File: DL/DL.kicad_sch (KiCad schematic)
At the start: 39 parts, among them IC1 MCP6V96UT-E_OT, IC2 SCD42-D-R2, IC3 TGS3870-B00, J3 SD_Card, J4 Conn_01x05_Male, J5 Conn_01x05_Male, J6 Conn_01x05_Male, J7 Conn_01x05_Male, Q1 BSS84, Q2 2N7002, U1 SHT31-DIS, U2 TGS5141-P00, U3 Pico

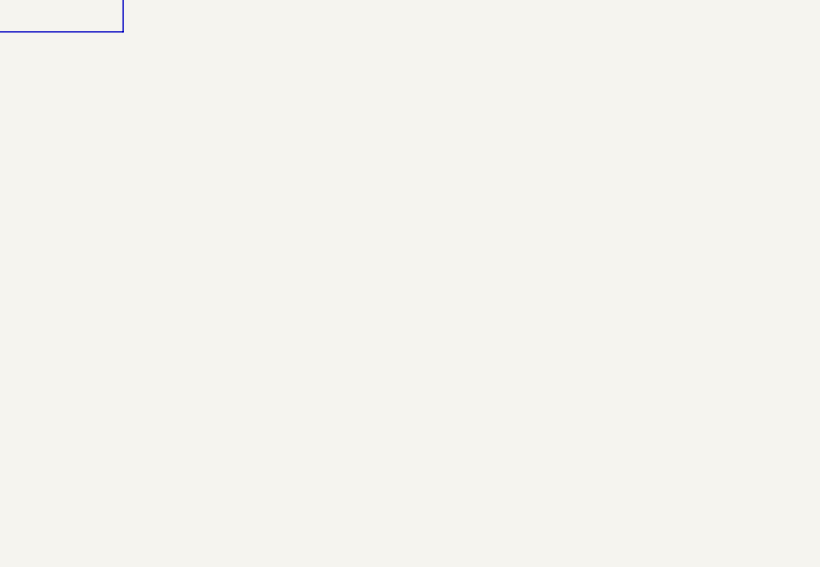
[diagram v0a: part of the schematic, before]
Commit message: Final PCB design
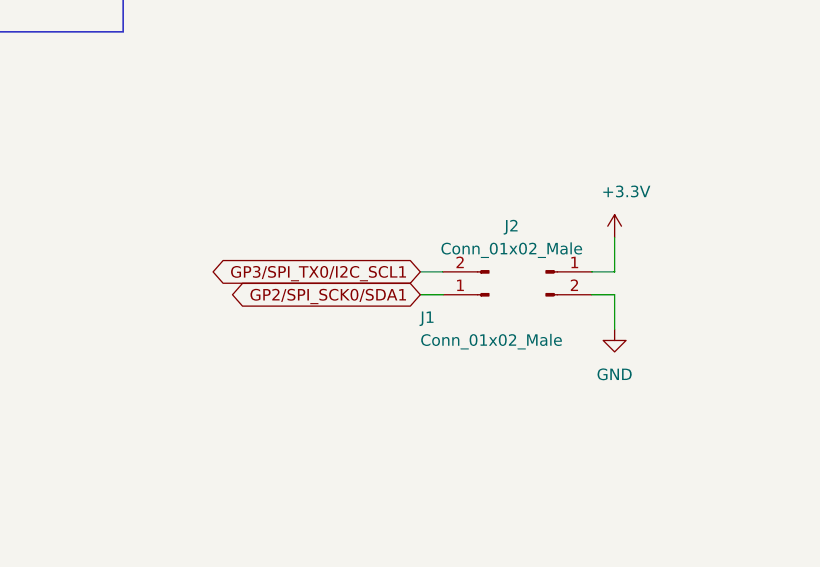
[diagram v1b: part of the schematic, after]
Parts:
- added J1, J2: Conn_01x02_Male, Connector_PinHeader_2.54mm:PinHeader_1x02_P2.54mm_Vertical, symbol Connector:Conn_01x02_Male
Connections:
- net +3.3V: now also J2.1 (Pin_1)
- net GND: now also J2.2 (Pin_2)
- net GP2/SPI_SCK0/SDA1: now also J1.1 (Pin_1)
- net GP3/SPI_TX0/I2C_SCL1: now also J1.2 (Pin_2)
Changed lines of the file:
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@@
+    (stroke (width 0) (type default) (color 0 0 0 0))
+  )
+  (wire (pts (xy 304.8 199.39) (xy 307.34 199.39))
     (stroke (width 0) (type default) (color 0 0 0 0))
   )
@@
     (stroke (width 0) (type default) (color 0 0 0 0))
   )
+  (wire (pts (xy 307.34 199.39) (xy 307.34 195.58))
+    (stroke (width 0) (type default) (color 0 0 0 0))
+  )
   (wire (pts (xy 276.86 58.42) (xy 279.4 58.42))
     (stroke (width 0) (type default) (color 0 0 0 0))
@@
     (stroke (width 0) (type default) (color 0 0 0 0))
   )
+  (wire (pts (xy 304.8 201.93) (xy 307.34 201.93))
+    (stroke (width 0) (type default) (color 0 0 0 0))
+  )
   (polyline (pts (xy 87.63 107.95) (xy 12.7 107.95))
     (stroke (width 0) (type default) (color 0 0 0 0))
@@
     (stroke (width 0) (type default) (color 0 0 0 0))
   )
+  (wire (pts (xy 285.75 199.39) (xy 288.29 199.39))
+    (stroke (width 0) (type default) (color 0 0 0 0))
+  )
   (wire (pts (xy 17.78 159.004) (xy 17.78 161.29))
     (stroke (width 0) (type default) (color 0 0 0 0))
@@
     (stroke (width 0) (type default) (color 0 0 0 0))
   )
+  (wire (pts (xy 285.75 201.93) (xy 288.29 201.93))
+    (stroke (width 0) (type default) (color 0 0 0 0))
+  )
   (wire (pts (xy 200.66 39.37) (xy 200.66 48.26))
     (stroke (width 0) (type default) (color 0 0 0 0))
@@
   )
   (wire (pts (xy 38.1 100.33) (xy 38.1 101.6))
+    (stroke (width 0) (type default) (color 0 0 0 0))
+  )
+  (wire (pts (xy 307.34 201.93) (xy 307.34 205.74))
     (stroke (width 0) (type default) (color 0 0 0 0))
   )
@@
     )
   )
+  (global_label "GP2{slash}SPI_SCK0{slash}SDA1" (shape bidirectional) (at 285.75 201.93 180) (fields_autoplaced)
+    (effects (font (size 1.27 1.27)) (justify right))
+    (property "Intersheet References" "${INTERSHEET_REFS}" (id 0) (at 263.1379 201.8506 0)
+      (effects (font (size 1.27 1.27)) (justify right) hide)
+    )
+  )
   (global_label "GP20{slash}I2C_SDA0" (shape bidirectional) (at 88.9 57.15 0) (fields_autoplaced)
     (effects (font (size 1.27 1.27)) (justify left))
@@
     )
   )
+  (global_label "GP3{slash}SPI_TX0{slash}I2C_SCL1" (shape bidirectional) (at 285.75 199.39 180) (fields_autoplaced)
+    (effects (font (size 1.27 1.27)) (justify right))
+    (property "Intersheet References" "${INTERSHEET_REFS}" (id 0) (at 260.7188 199.3106 0)
+      (effects (font (size 1.27 1.27)) (justify right) hide)
+    )
+  )
   (global_label "GP22" (shape bidirectional) (at 88.9 49.53 0) (fields_autoplaced)
     (effects (font (size 1.27 1.27)) (justify left))
@@
     (pin "1")
     (pin "2")
+  )
+  (symbol (lib_id "power:GND") (at 307.34 205.74 0) (unit 1)
+    (in_bom yes) (on_board yes) (fields_autoplaced)
+    (property "Reference" "#PWR014" (id 0) (at 307.34 212.09 0)
+      (effects (font (size 1.27 1.27)) hide)
+    )
+    (property "Value" "GND" (id 1) (at 307.34 210.82 0))
+    (property "Footprint" "" (id 2) (at 307.34 205.74 0)
+      (effects (font (size 1.27 1.27)) hide)
+    )
+    (property "Datasheet" "" (id 3) (at 307.34 205.74 0)
+      (effects (font (size 1.27 1.27)) hide)
+    )
+    (pin "1")
   )
   (symbol (lib_id "Transistor_FET:2N7002") (at 359.41 57.15 0) (unit 1)
@@
     (pin "1")
   )
+  (symbol (lib_id "Connector:Conn_01x02_Male") (at 299.72 199.39 0) (unit 1)
+    (in_bom yes) (on_board yes)
+    (property "Reference" "J2" (id 0) (at 295.91 194.31 0))
+    (property "Value" "Conn_01x02_Male" (id 1) (at 295.91 196.85 0))
+    (property "Footprint" "Connector_PinHeader_2.54mm:PinHeader_1x02_P2.54mm_Vertical" (id 2) (at 299.72 199.39 0)
+      (effects (font (size 1.27 1.27)) hide)
+    )
+    (property "Datasheet" "~" (id 3) (at 299.72 199.39 0)
+      (effects (font (size 1.27 1.27)) hide)
+    )
+    (pin "1")
+    (pin "2")
+  )
   (symbol (lib_id "power:GND") (at 332.74 152.4 0) (unit 1)
     (in_bom yes) (on_board yes) (fields_autoplaced)
@@
     (pin "2")
   )
+  (symbol (lib_id "power:+3.3V") (at 307.34 195.58 0) (unit 1)
+    (in_bom yes) (on_board yes)
+    (property "Reference" "#PWR013" (id 0) (at 307.34 199.39 0)
+      (effects (font (size 1.27 1.27)) hide)
+    )
+    (property "Value" "+3.3V" (id 1) (at 308.61 190.5 0))
+    (property "Footprint" "" (id 2) (at 307.34 195.58 0)
+      (effects (font (size 1.27 1.27)) hide)
+    )
+    (property "Datasheet" "" (id 3) (at 307.34 195.58 0)
+      (effects (font (size 1.27 1.27)) hide)
+    )
+    (pin "1")
+  )
   (symbol (lib_id "power:GND") (at 38.1 101.6 0) (unit 1)
     (in_bom yes) (on_board yes) (fields_autoplaced)
@@
     )
     (pin "1")
+  )
+  (symbol (lib_id "Connector:Conn_01x02_Male") (at 293.37 201.93 180) (unit 1)
+    (in_bom yes) (on_board yes)
+    (property "Reference" "J1" (id 0) (at 285.75 204.47 0)
+      (effects (font (size 1.27 1.27)) (justify right))
+    )
+    (property "Value" "Conn_01x02_Male" (id 1) (at 285.75 207.01 0)
+      (effects (font (size 1.27 1.27)) (justify right))
+    )
+    (property "Footprint" "Connector_PinHeader_2.54mm:PinHeader_1x02_P2.54mm_Vertical" (id 2) (at 293.37 201.93 0)
+      (effects (font (size 1.27 1.27)) hide)
+    )
+    (property "Datasheet" "~" (id 3) (at 293.37 201.93 0)
+      (effects (font (size 1.27 1.27)) hide)
+    )
+    (pin "1")
+    (pin "2")
   )
   (symbol (lib_id "power:GND") (at 377.19 67.31 0) (unit 1)
@@
       (reference "#PWR012") (unit 1) (value "GND") (footprint "")
     )
+    (path "/917253d4-830e-4676-bd08-7cea5380aeca"
+      (reference "#PWR013") (unit 1) (value "+3.3V") (footprint "")
+    )
+    (path "/0b7ad6f7-466a-4bc5-b0cd-832825c5104c"
+      (reference "#PWR014") (unit 1) (value "GND") (footprint "")
+    )
     (path "/4e6550f9-a20e-4af4-b2a9-5f355a33d960"
       (reference "#PWR0101") (unit 1) (value "GND") (footprint "")
@@
       (reference "IC3") (unit 1) (value "TGS3870-B00") (footprint "TGS3870-B00:TGS3870B00")
     )
+    (path "/a33771af-3110-4c71-81b7-4d80190bce44"
+      (reference "J1") (unit 1) (value "Conn_01x02_Male") (footprint "Connector_PinHeader_2.54mm:PinHeader_1x02_P2.54mm_Vertical")
+    )
+    (path "/53770f53-83c7-4934-95c6-04d6a107de5f"
+      (reference "J2") (unit 1) (value "Conn_01x02_Male") (footprint "Connector_PinHeader_2.54mm:PinHeader_1x02_P2.54mm_Vertical")
+    )
     (path "/300aa512-2f66-4c26-a530-50c091b3a099"
